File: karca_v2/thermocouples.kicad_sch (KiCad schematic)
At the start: 17 parts, among them J7 Screw_Terminal_01x08

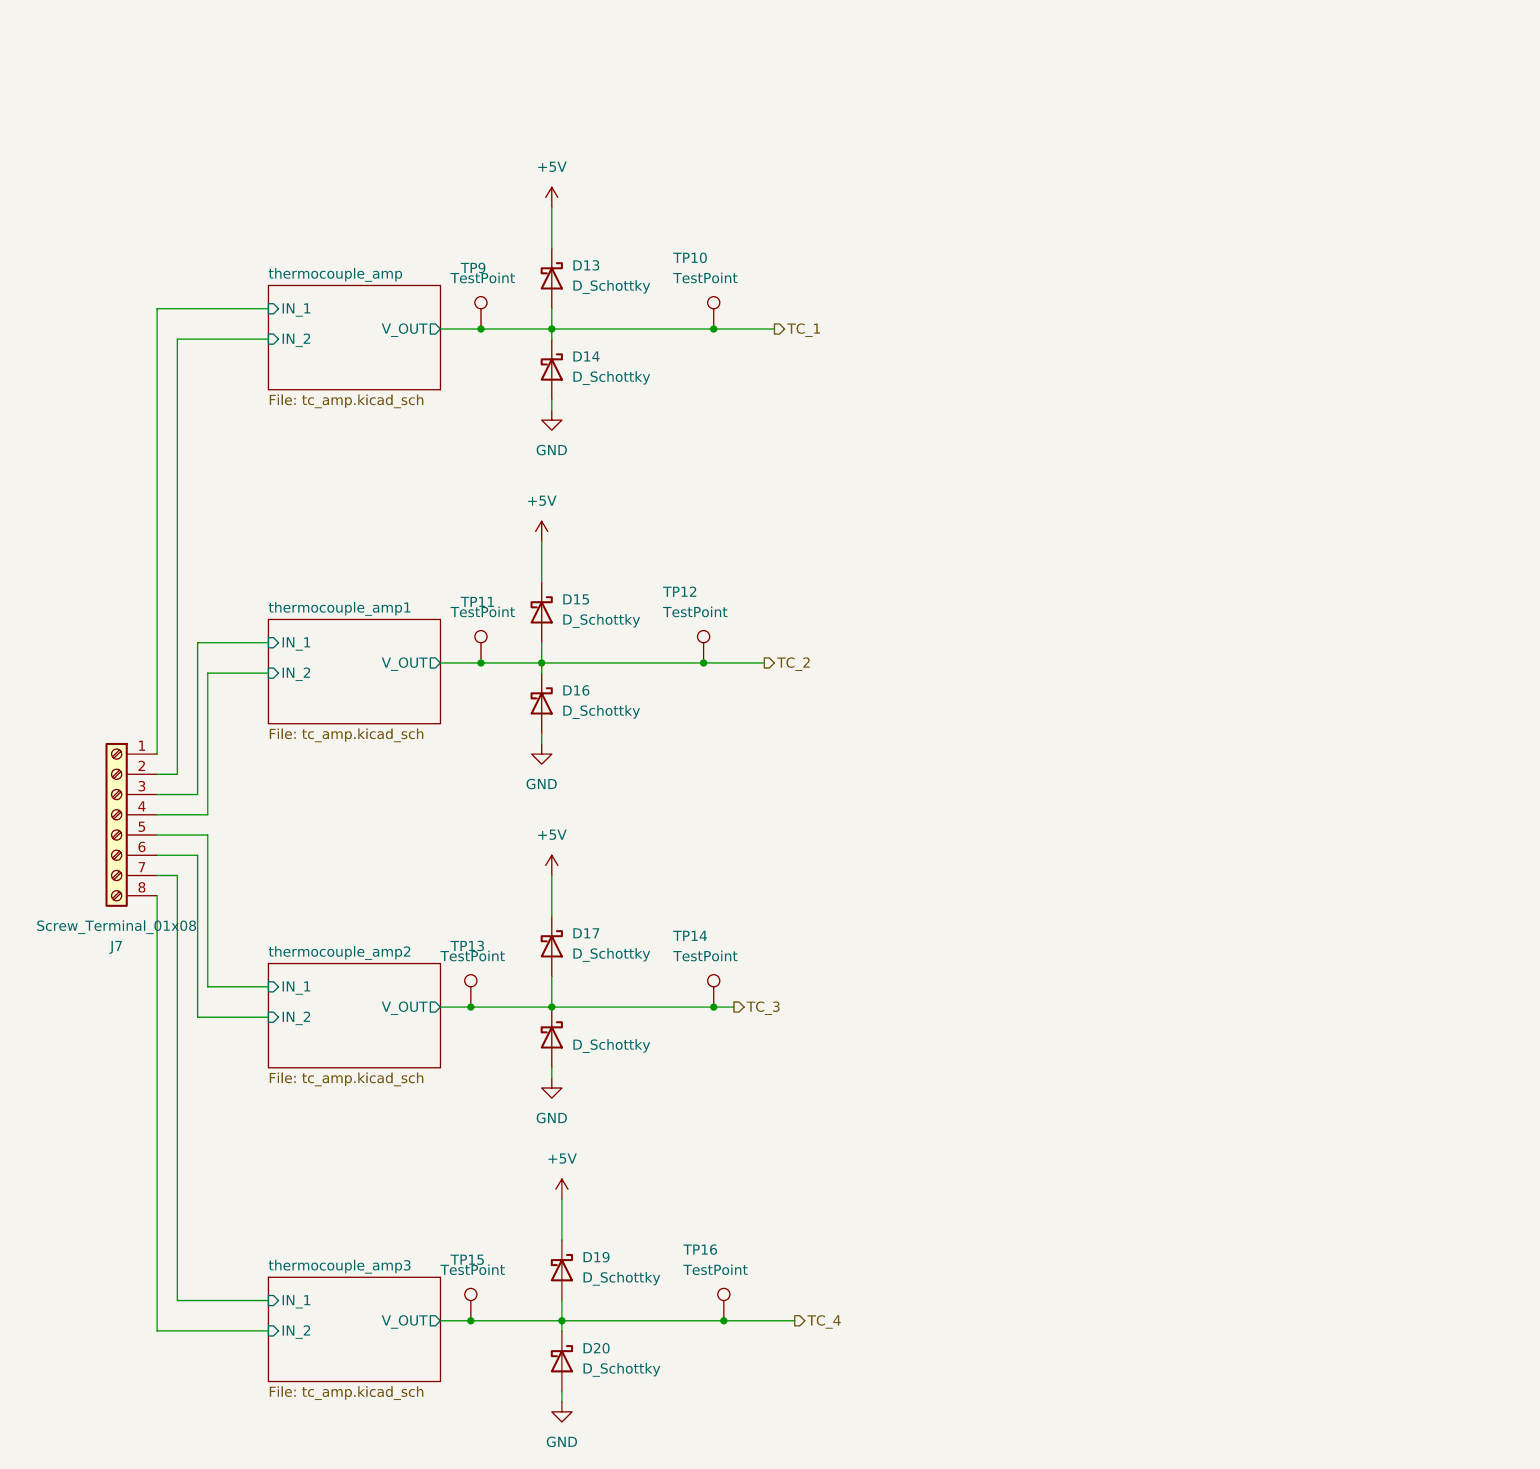
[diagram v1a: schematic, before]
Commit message: updated
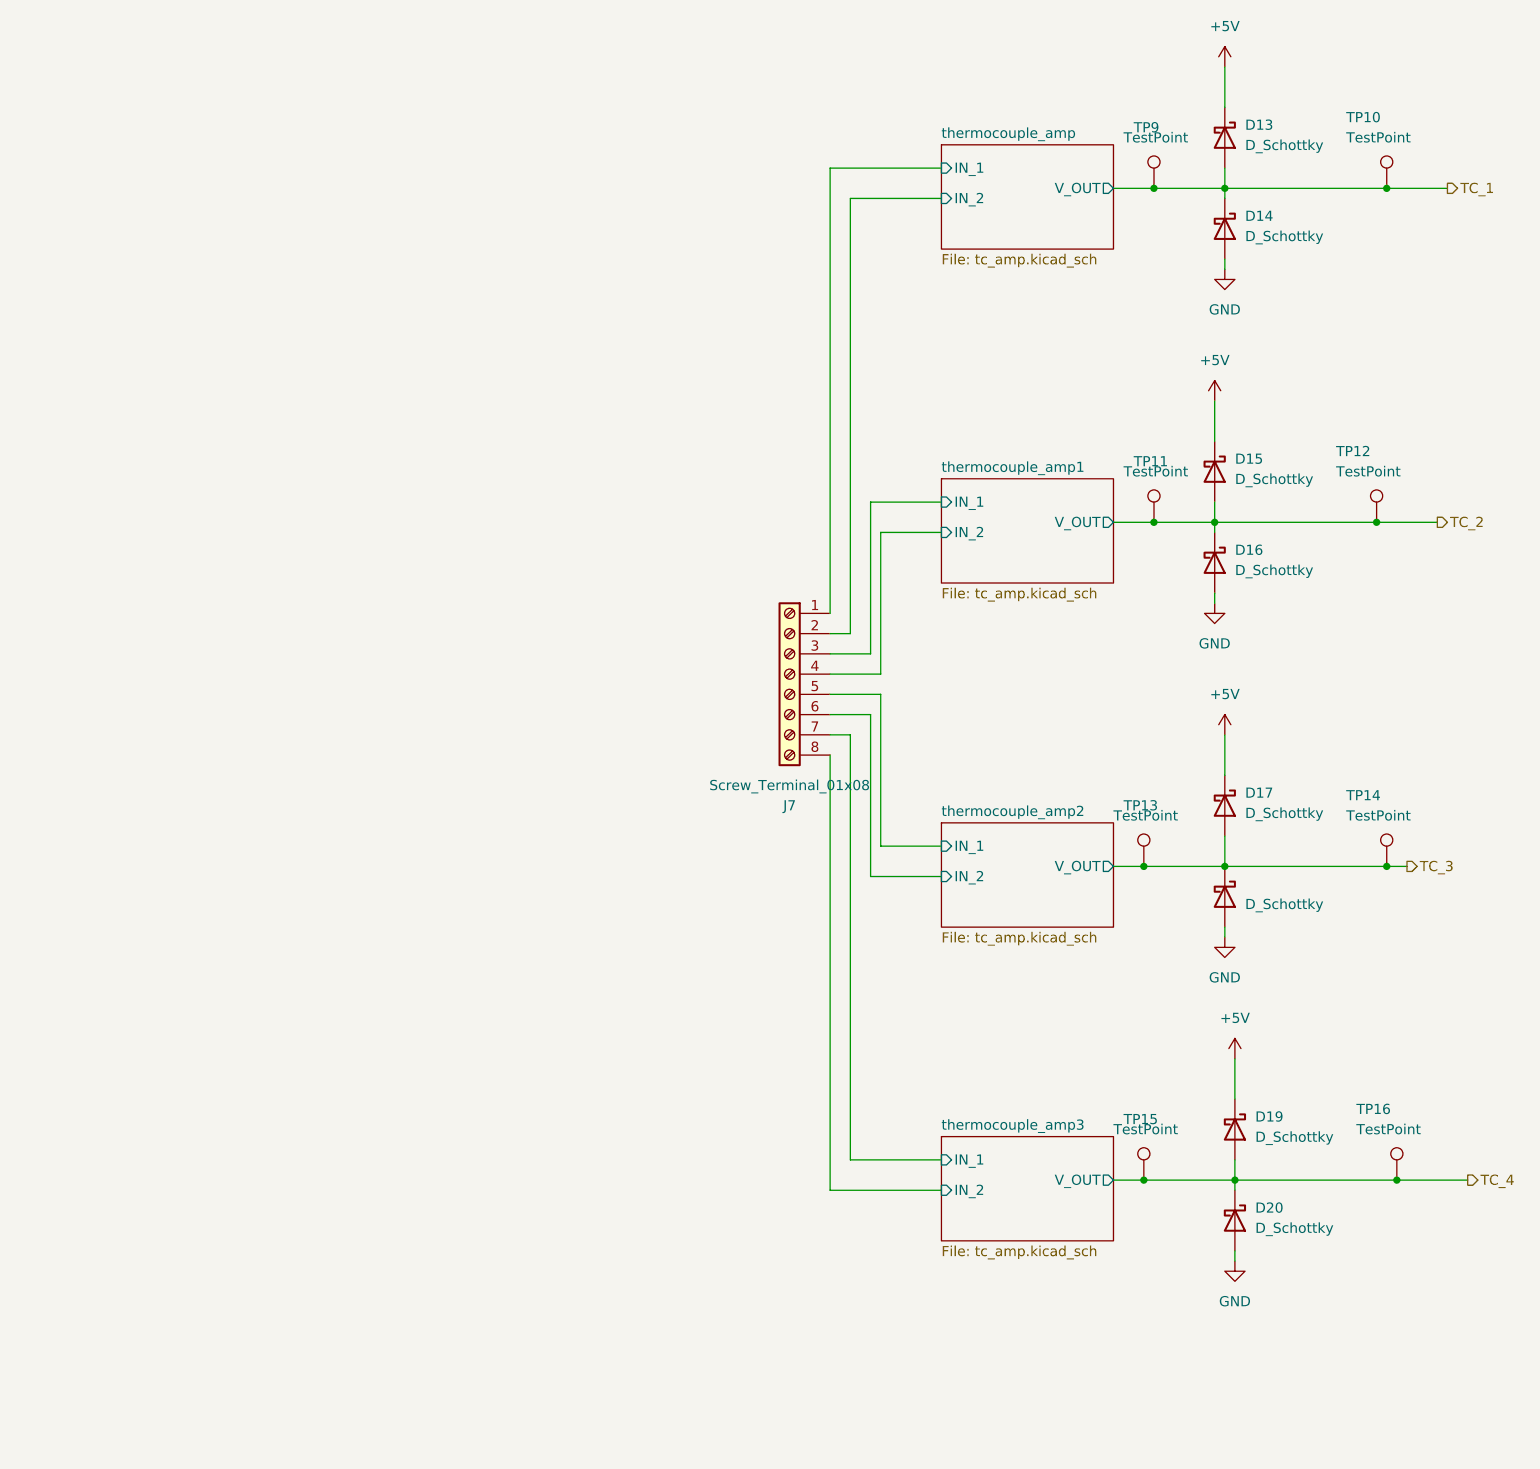
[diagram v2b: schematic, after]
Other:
- moved on the sheet: D13, D14, D15, D16, D17, D19, D20, J7, TP10, TP11, TP12, TP13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
